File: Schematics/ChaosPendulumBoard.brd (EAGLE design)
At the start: 30.5 x 85.1 mm, 6 parts, among them IC1 TEENSY_3.2_NO_BOTTOM

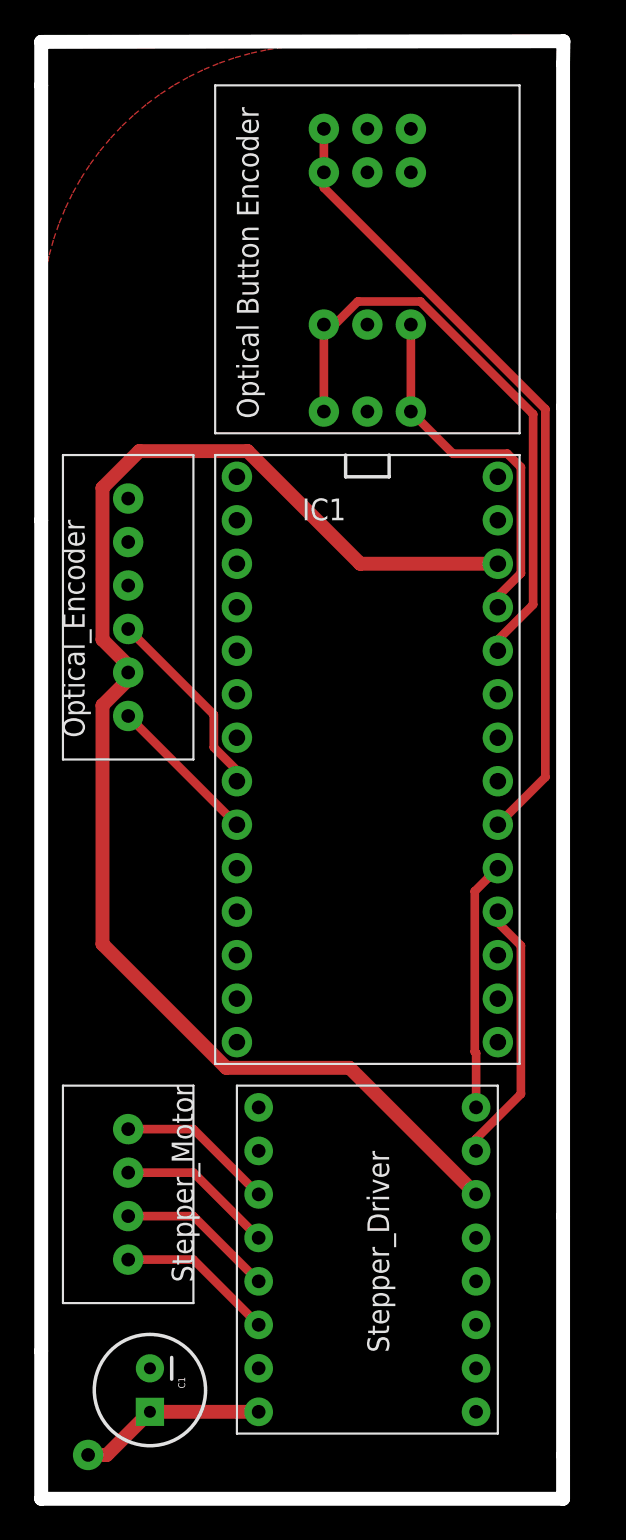
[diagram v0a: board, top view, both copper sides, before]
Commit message: Finished optimization
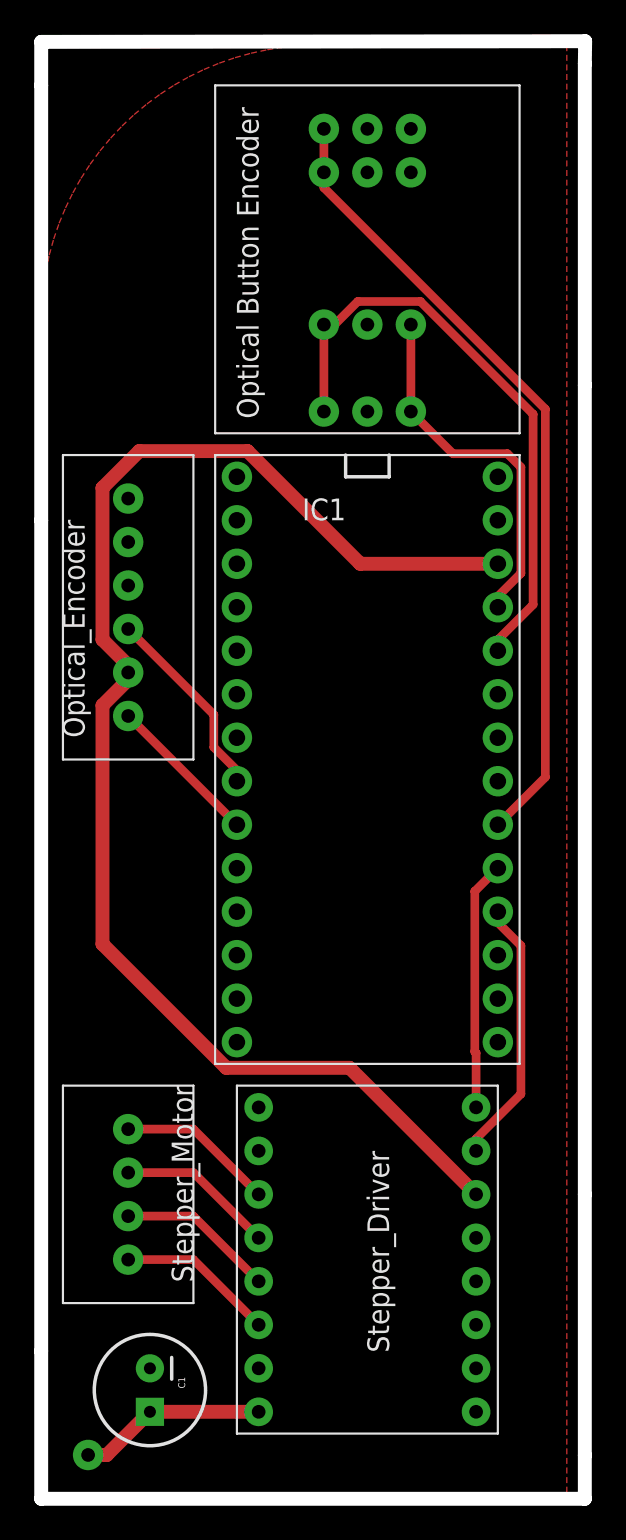
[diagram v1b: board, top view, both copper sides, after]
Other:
- board size 30.5 x 85.1 mm -> 31.8 x 85.1 mm
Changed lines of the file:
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@@
 <board>
 <plain>
-<wire x1="20.34" y1="10.2" x2="-10.16" y2="10.16" width="0.8128" layer="20"/>
+<wire x1="21.61" y1="10.2" x2="-10.16" y2="10.16" width="0.8128" layer="20"/>
 <wire x1="-10.16" y1="10.16" x2="-10.16" y2="7.62" width="0.8128" layer="20"/>
 <wire x1="-10.16" y1="7.62" x2="-10.16" y2="-17.78" width="0.8128" layer="20"/>
 <wire x1="-10.16" y1="-17.78" x2="-10.16" y2="-66.31" width="0.8128" layer="20"/>
 <wire x1="-10.16" y1="-66.31" x2="-10.16" y2="-74.93" width="0.8128" layer="20"/>
-<wire x1="-10.16" y1="-74.93" x2="20.32" y2="-74.93" width="0.8128" layer="20"/>
-<wire x1="20.32" y1="-74.93" x2="20.32" y2="-72.39" width="0.8128" layer="20"/>
-<wire x1="20.32" y1="-72.39" x2="20.32" y2="-58.42" width="0.8128" layer="20"/>
-<wire x1="20.32" y1="-58.42" x2="20.32" y2="-11.16" width="0.8128" layer="20"/>
-<wire x1="20.32" y1="-11.16" x2="20.32" y2="8.89" width="0.8128" layer="20"/>
-<wire x1="20.32" y1="8.89" x2="20.34" y2="10.2" width="0.8128" layer="20"/>
+<wire x1="-10.16" y1="-74.93" x2="21.59" y2="-74.93" width="0.8128" layer="20"/>
+<wire x1="21.59" y1="-74.93" x2="21.59" y2="-72.39" width="0.8128" layer="20"/>
+<wire x1="21.59" y1="-72.39" x2="21.59" y2="-57.15" width="0.8128" layer="20"/>
+<wire x1="21.59" y1="-57.15" x2="21.59" y2="-9.89" width="0.8128" layer="20"/>
+<wire x1="21.59" y1="-9.89" x2="21.59" y2="8.89" width="0.8128" layer="20"/>
+<wire x1="21.59" y1="8.89" x2="21.61" y2="10.2" width="0.8128" layer="20"/>
 </plain>
 <attributes>
